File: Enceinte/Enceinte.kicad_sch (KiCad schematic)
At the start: 18 parts, among them J1 Conn_01x07, J2 Conn_01x02, J3 Conn_01x02, J4 Conn_01x02, J5 Conn_01x02, J7 Conn_01x06, J8 Conn_01x02, J9 Conn_01x02, U1 L7805

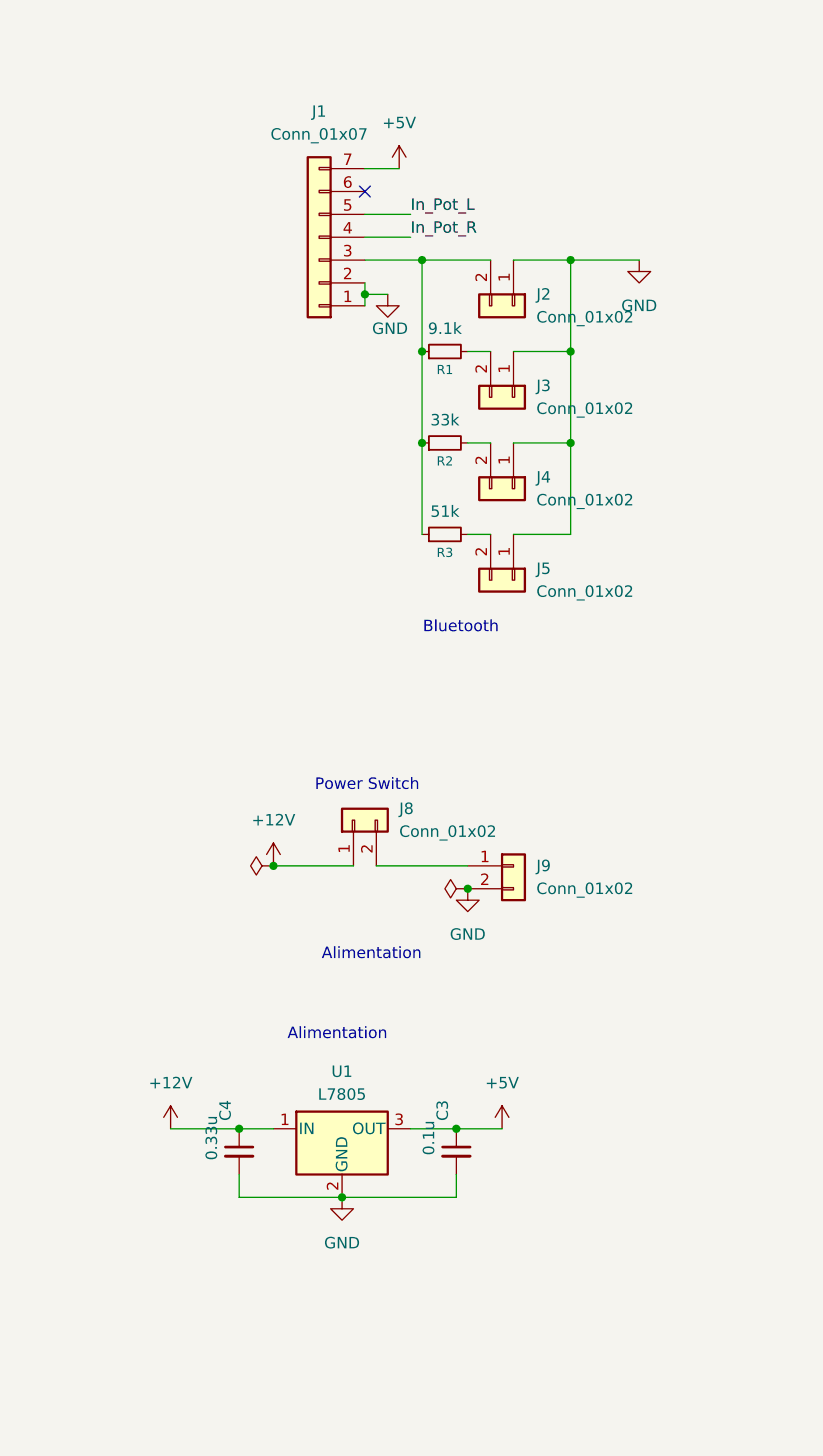
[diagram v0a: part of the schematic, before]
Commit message: des changements sont à faire
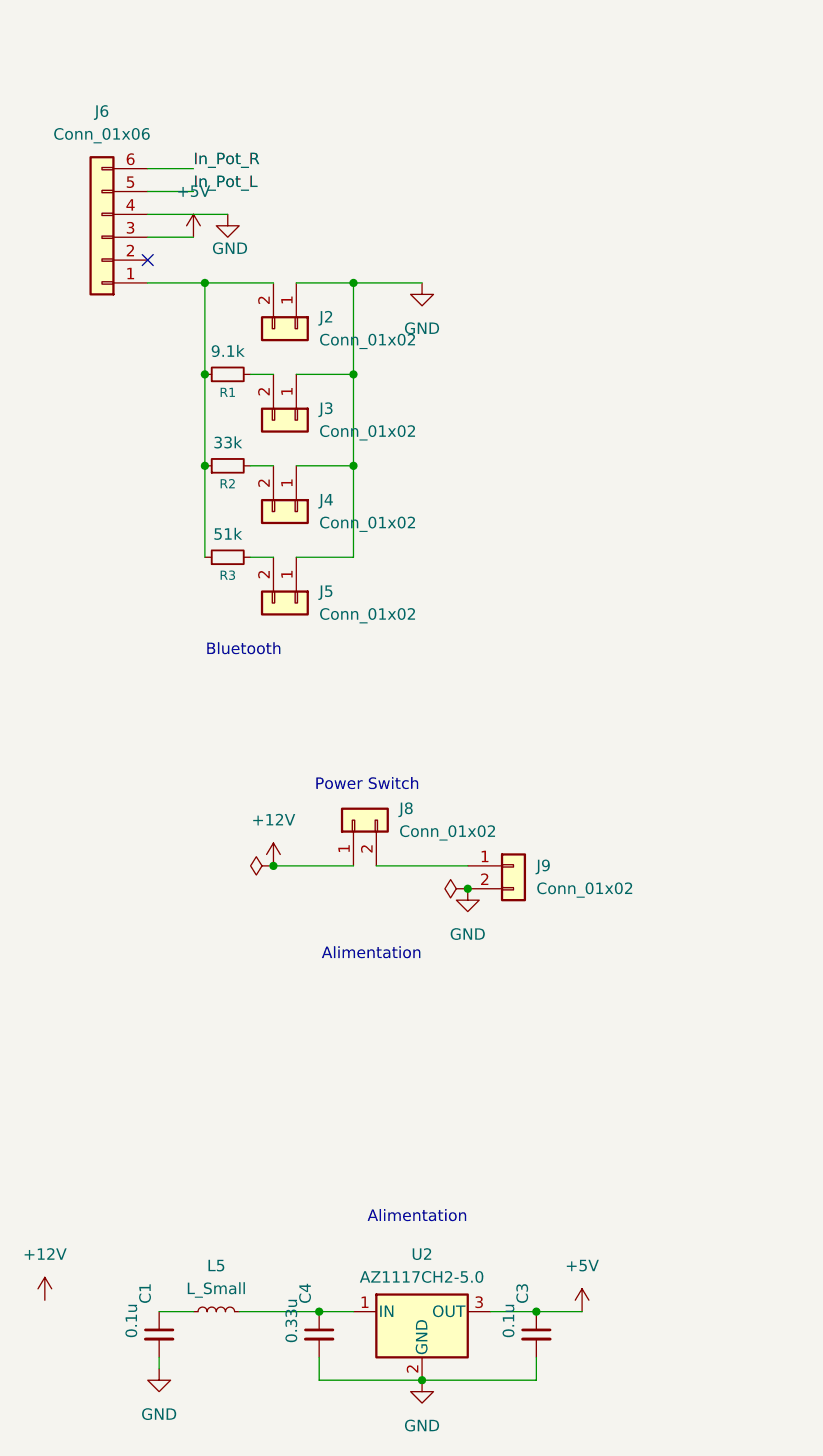
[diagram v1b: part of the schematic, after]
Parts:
- removed J1: Conn_01x07, Connector_PinSocket_2.54mm:PinSocket_1x07_P2.54mm_Vertical, symbol Connector_Generic:Conn_01x07
- removed U1: L7805, L7805:TO255P1020X450X2000-3, symbol Regulator_Linear:L7805
- added C1: 0.1u, Capacitor_SMD:C_0603_1608Metric, symbol Device:C_Small
- added J6: Conn_01x06, Connector_PinSocket_2.54mm:PinSocket_1x06_P2.54mm_Vertical, symbol Connector_Generic:Conn_01x06
- added L5: L_Small, symbol Device:L_Small
- added U2: AZ1117CH2-5.0, Package_TO_SOT_SMD:SOT-223-3_TabPin2, symbol Regulator_Linear:AZ1117CH2-5.0
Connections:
- net +12V: no longer C4.1
- net +5V: now also J6.3 (Pin_3), U2.3 (OUT)
- net GND: now also C1.2, J6.4 (Pin_4), U2.2 (GND)
- net In_Pot_L: now also J6.5 (Pin_5)
- net In_Pot_R: now also J6.6 (Pin_6)
- net at J2.2 (Pin_2), R1.1, R2.1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: now also J6.1 (Pin_1)
- new net: C1.1, L5.1
- new net: C4.1, L5.2, U2.1 (IN)
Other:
- moved on the sheet: C3, C4, J2, J3, J4, J5, R1, R2, R3

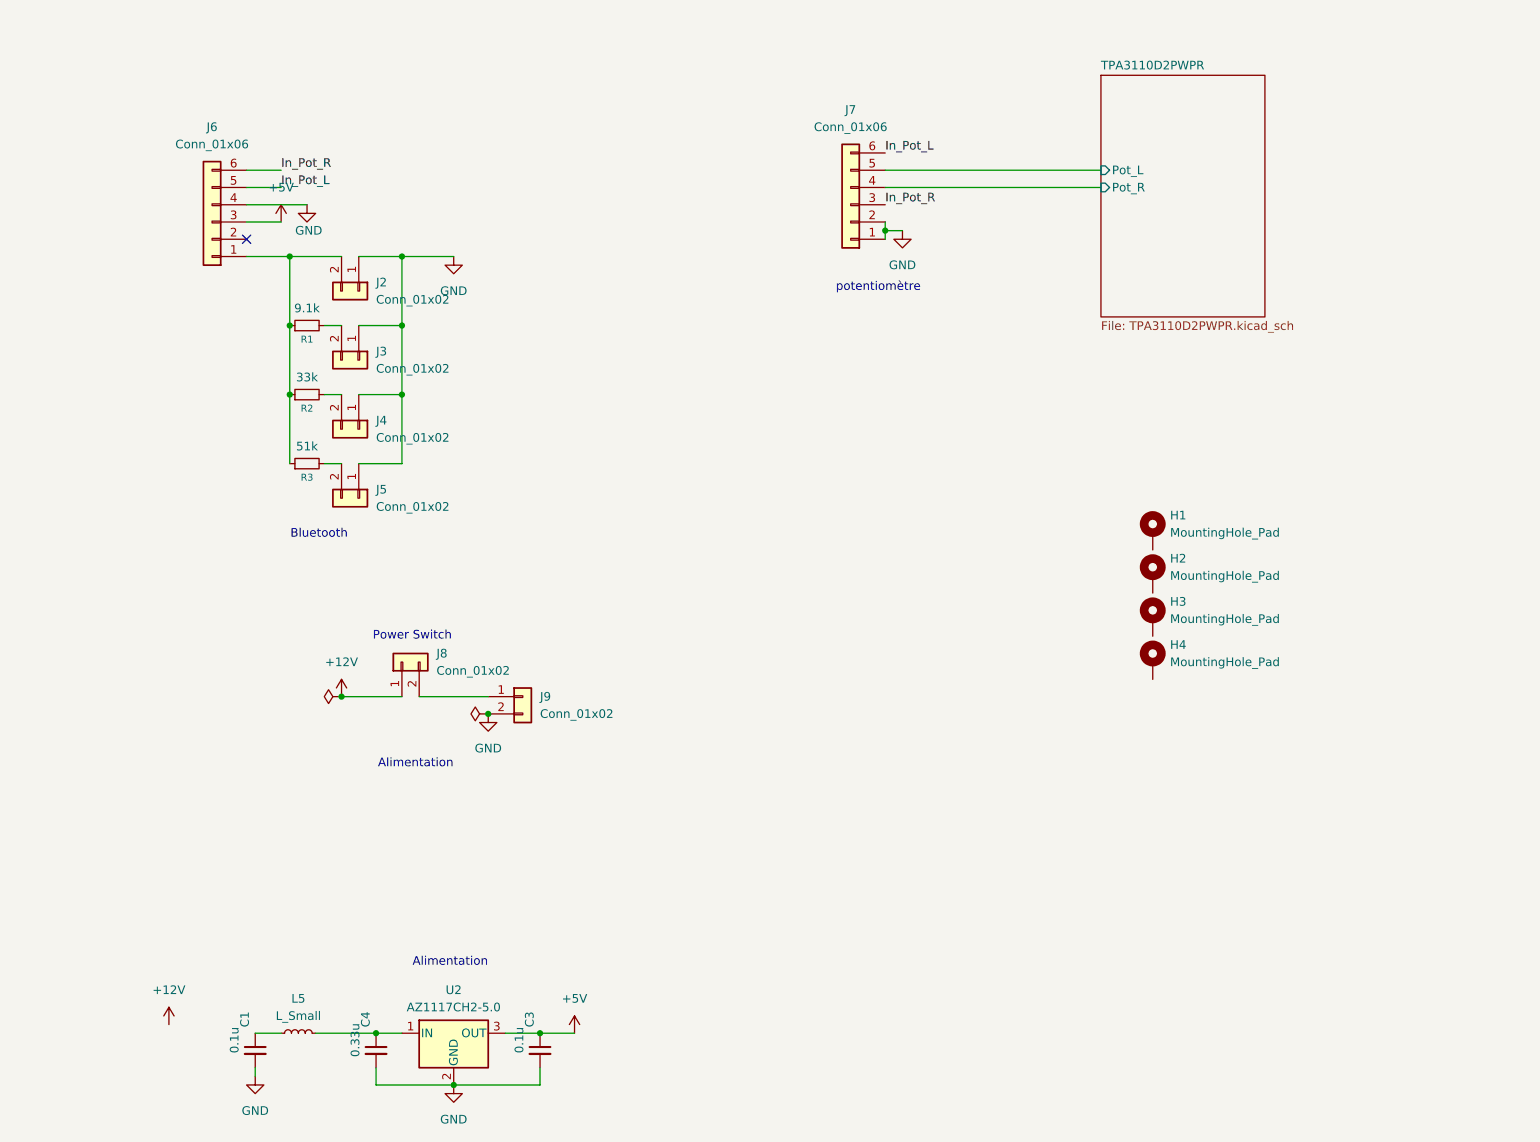
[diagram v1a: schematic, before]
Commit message: doc latex
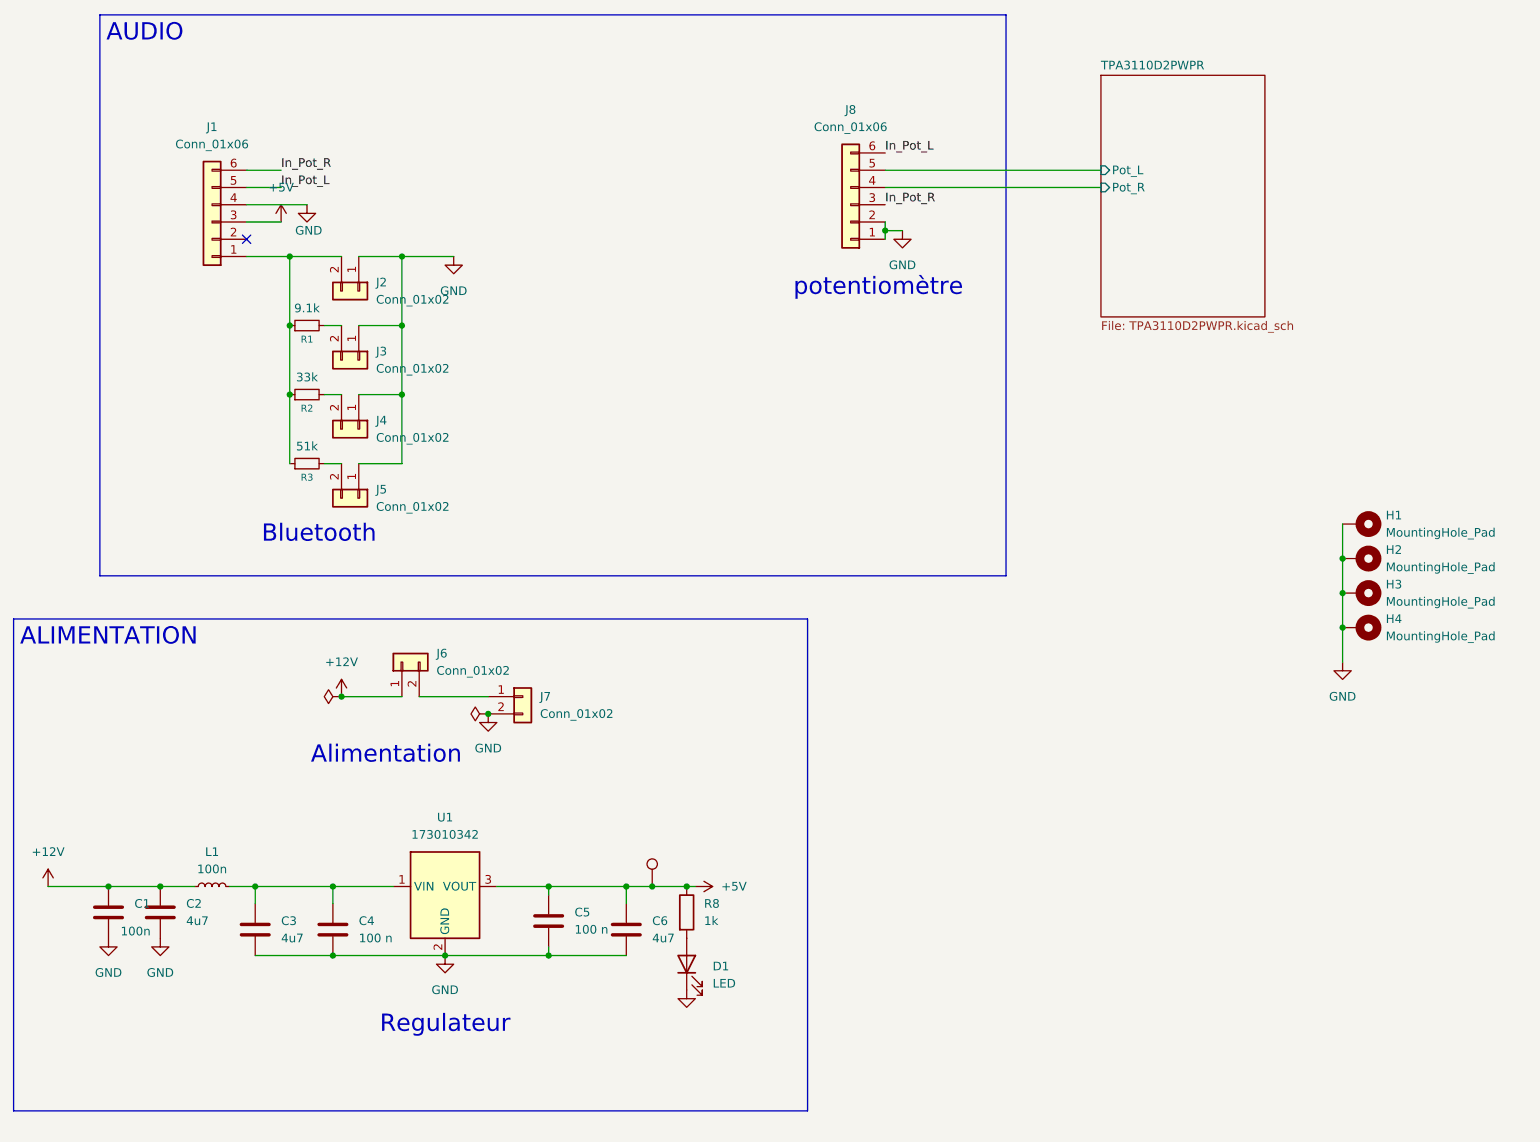
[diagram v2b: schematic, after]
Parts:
- removed C1, C3: 0.1u, Capacitor_SMD:C_0603_1608Metric, symbol Device:C_Small
- removed C4: 0.33u, Capacitor_SMD:C_0603_1608Metric, symbol Device:C_Small
- removed L5: L_Small, symbol Device:L_Small
- removed U2: AZ1117CH2-5.0, Package_TO_SOT_SMD:SOT-223-3_TabPin2, symbol Regulator_Linear:AZ1117CH2-5.0
- added C1: 100n, Capacitor_SMD:C_0603_1608Metric, symbol Device:C
- added C2, C3, C6: 4u7, Capacitor_SMD:C_0603_1608Metric, symbol Device:C
- added C4, C5: 100 n, Capacitor_SMD:C_0603_1608Metric, symbol Device:C
- added D1: LED, LED_SMD:LED_0603_1608Metric, symbol Device:LED
- added L1: 100n, Inductor_SMD:L_0603_1608Metric, symbol Device:L_Small
- added R8: 1k, Resistor_SMD:R_0402_1005Metric, symbol Device:R
- added TP1: TestPoint, TestPoint:TestPoint_Pad_D1.5mm, symbol Connector:TestPoint
- added U1: 173010342, MagIC_THT_Wurth:U_Wurth_MagIC-FDSM_173010x42, symbol MagIC_Wurth_MagIC-FDSM:173010342
- J1: renamed from J6; footprint Connector_PinSocket_2.54mm:PinSocket_1x06_P2.54mm_Vertical -> Connector_JST:JST_XH_B6B-XH-A_1x06_P2.50mm_Vertical
- J2, J3, J4, J5: footprint Connector_PinSocket_2.54mm:PinSocket_1x02_P2.54mm_Vertical -> Connector_JST:JST_XH_B2B-XH-A_1x02_P2.50mm_Vertical
- J6: renamed from J8; footprint Connector_PinSocket_2.54mm:PinSocket_1x02_P2.54mm_Vertical -> Connector_JST:JST_XH_B2B-XH-A_1x02_P2.50mm_Vertical
- J7: renamed from J9; footprint Connector_PinSocket_2.54mm:PinSocket_1x02_P2.54mm_Vertical -> Connector_JST:JST_XH_B2B-XH-A_1x02_P2.50mm_Vertical
- J8: renamed from J7; footprint Connector_PinSocket_2.54mm:PinSocket_1x06_P2.54mm_Vertical -> Connector_JST:JST_XH_B6B-XH-A_1x06_P2.50mm_Vertical
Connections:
- net +12V: now also C1.2, C2.1, L1.1
- net +5V: now also C5.1, C6.1, R8.1, TP1.1, U1.3 (VOUT)
- net GND: now also H1.1, H2.1, H3.1, H4.1, C1.1, C2.2, C3.2, C4.2, C5.2, C6.2, D1.1 (K), U1.2 (GND)
- new net: C3.1, C4.1, L1.2, U1.1 (VIN)
- new net: D1.2 (A), R8.2
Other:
- note added: "Regulateur"
- note removed: "Power Switch"
- moved on the sheet: H1, H2, H3, H4

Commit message: nouvelles inductances
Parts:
- L1: footprint Inductor_SMD:L_0603_1608Metric -> Library_inductance_new:CWF1612A100J
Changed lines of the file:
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@@
 			)
 		)
-		(property "Footprint" "Inductor_SMD:L_0603_1608Metric"
+		(property "Footprint" "Library_inductance_new:CWF1612A100J"
 			(at 45.72 151.13 0)
 			(effects
